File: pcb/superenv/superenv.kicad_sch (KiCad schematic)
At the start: 29 parts, among them J1 TYPE-C-31-M-04, J2 Power-Header, J3 UART, J4 I2C, J5 I2C, J6 SGP41BB, J7 SCD41BB, J8 AHT20+BMP280BB, U1 ESP32-C6-WROOM-1, U2 AMS1117-3.3, U3 DS18B20, U4 DS18B20, U5 DS18B20

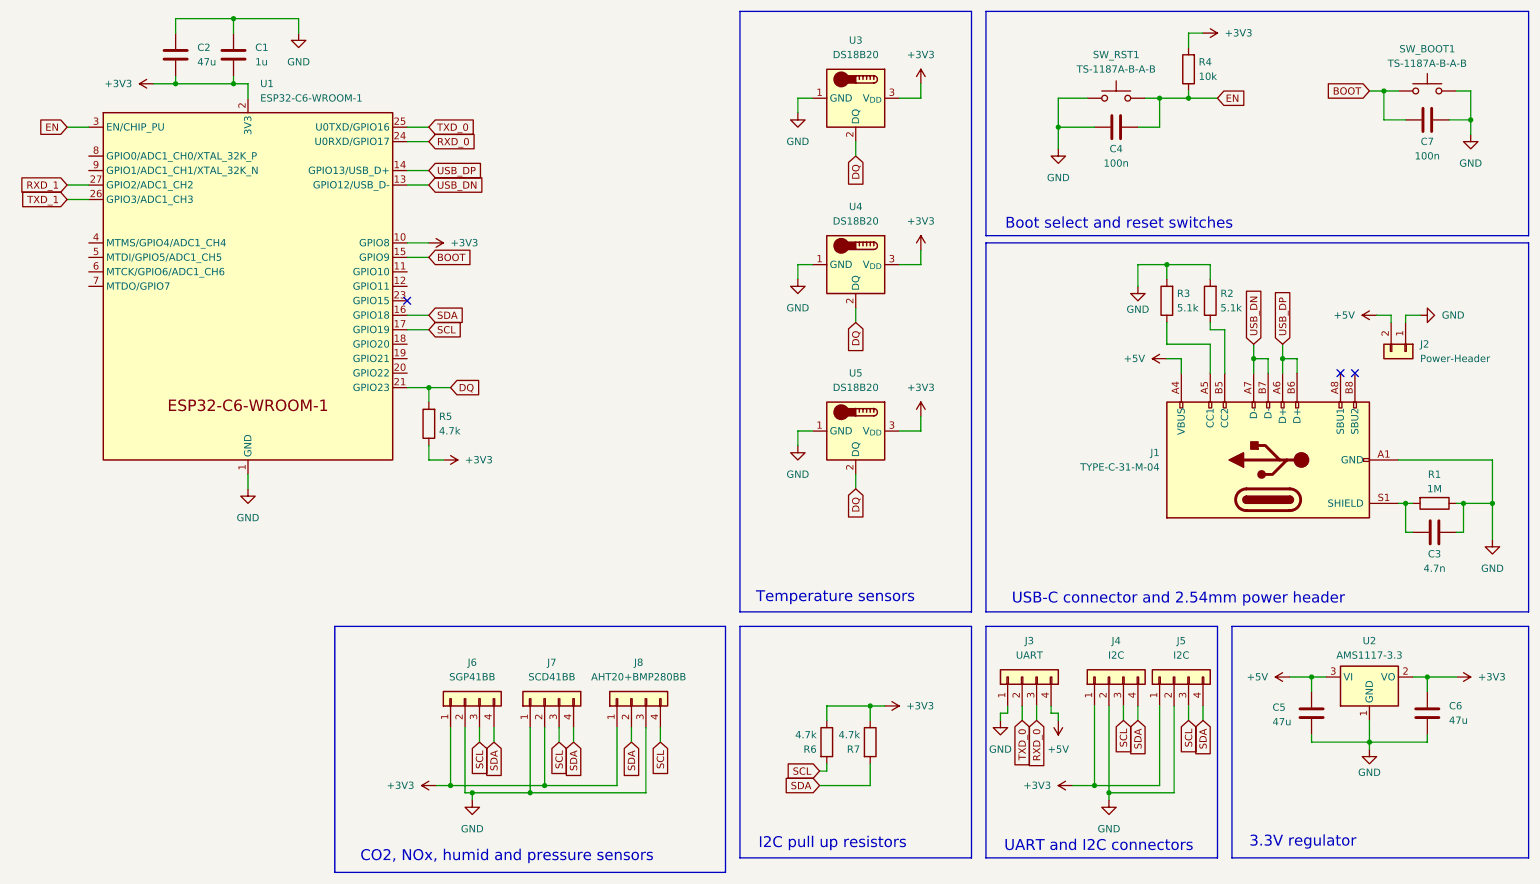
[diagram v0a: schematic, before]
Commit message: Add stuff
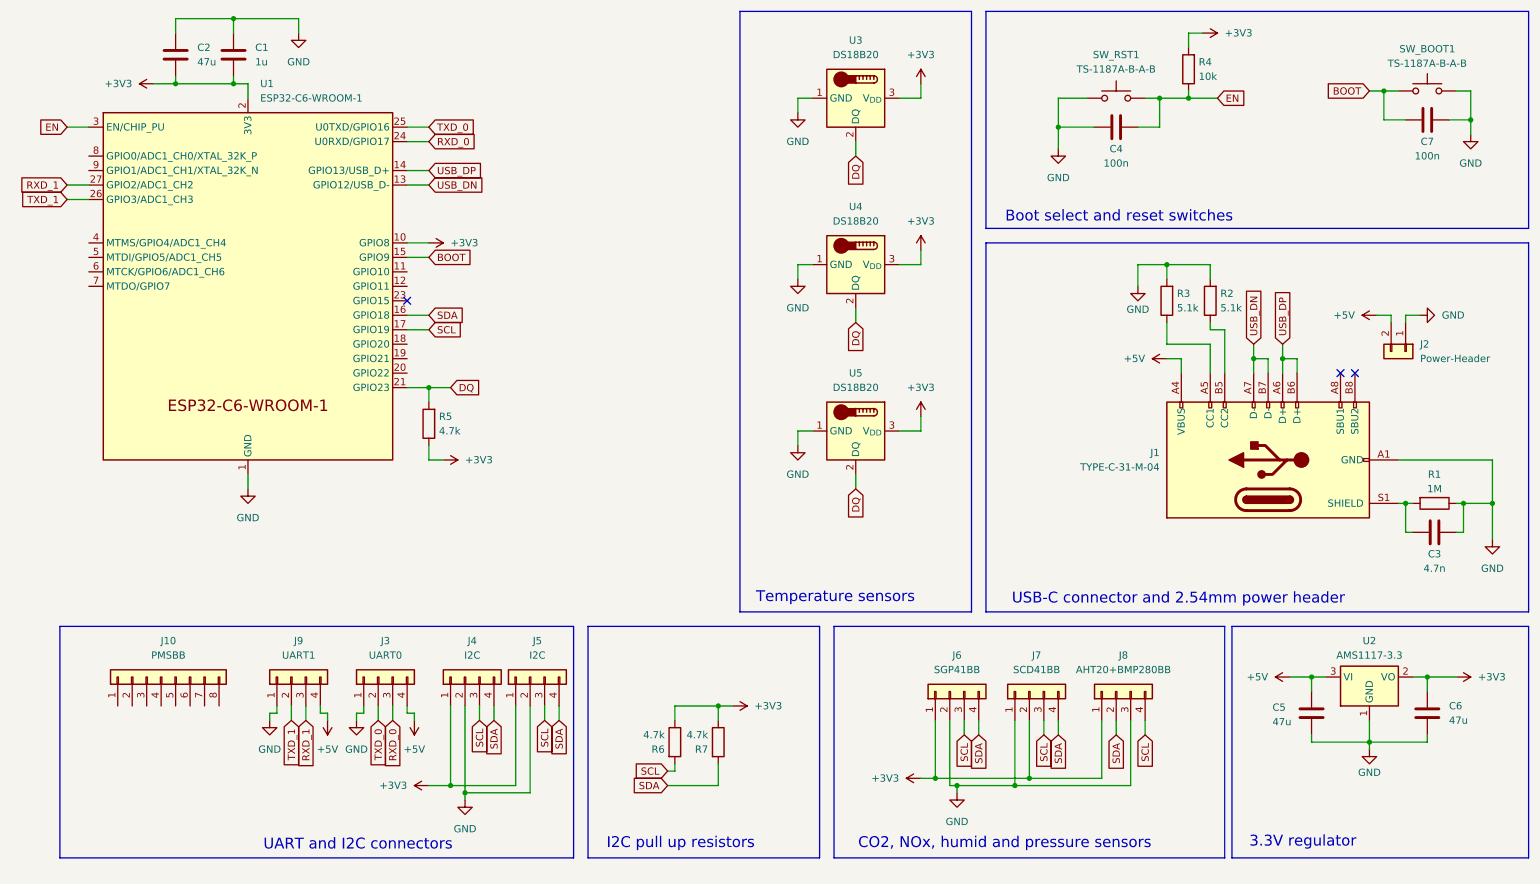
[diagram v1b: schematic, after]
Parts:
- added J10: PMSBB, Connector_JST:JST_GH_BM08B-GHS-TBT_1x08-1MP_P1.25mm_Vertical, symbol Connector_Generic:Conn_01x08
- added J9: UART1, Connector_PinHeader_2.54mm:PinHeader_1x04_P2.54mm_Vertical, symbol Connector_Generic:Conn_01x04
- J3: value UART -> UART0
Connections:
- net +5V: now also J9.4 (Pin_4)
- net GND: now also J9.1 (Pin_1)
- net RXD_1: now also J9.3 (Pin_3)
- net TXD_1: now also J9.2 (Pin_2)
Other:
- moved on the sheet: J3, J4, J5, J6, J7, J8, R6, R7
